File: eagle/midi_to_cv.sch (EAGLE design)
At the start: 46 parts, among them IC2 4504N, IC3 4099N, U1 ATMEGA328P_PDIP

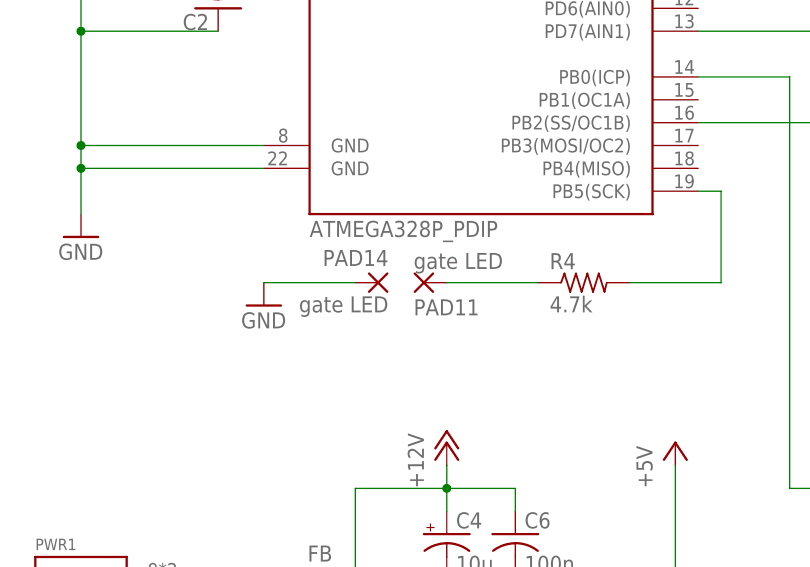
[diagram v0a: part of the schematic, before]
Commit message: cutout
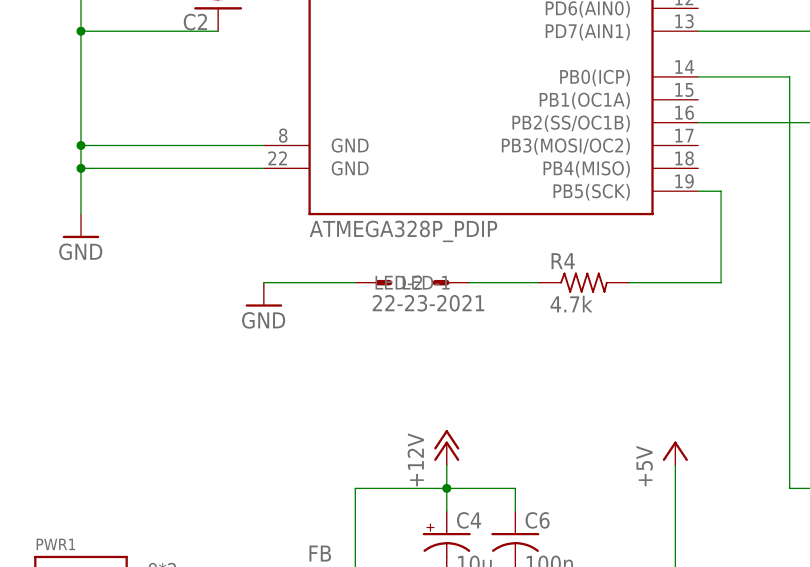
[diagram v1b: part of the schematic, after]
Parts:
- removed PAD11, PAD14: gate LED, wirepad:2,54/0,9
- added LED: 22-23-2021, con-molex:22-23-2021
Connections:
- removed net N$26: C4.-, C5.-, C6.2, C7.2, PWR1.GND
- net GND: now also C4.-, C5.-, C6.2, C7.2, LED-1.S, PWR1.GND; no longer PAD14.P
- net N$11: now also LED-2.S; no longer PAD11.P
